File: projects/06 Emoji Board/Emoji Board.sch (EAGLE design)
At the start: 25 parts, among them M2 MAX7219, U2 ATMEGA8A-AU-TQFP32, Y1 16MHZ

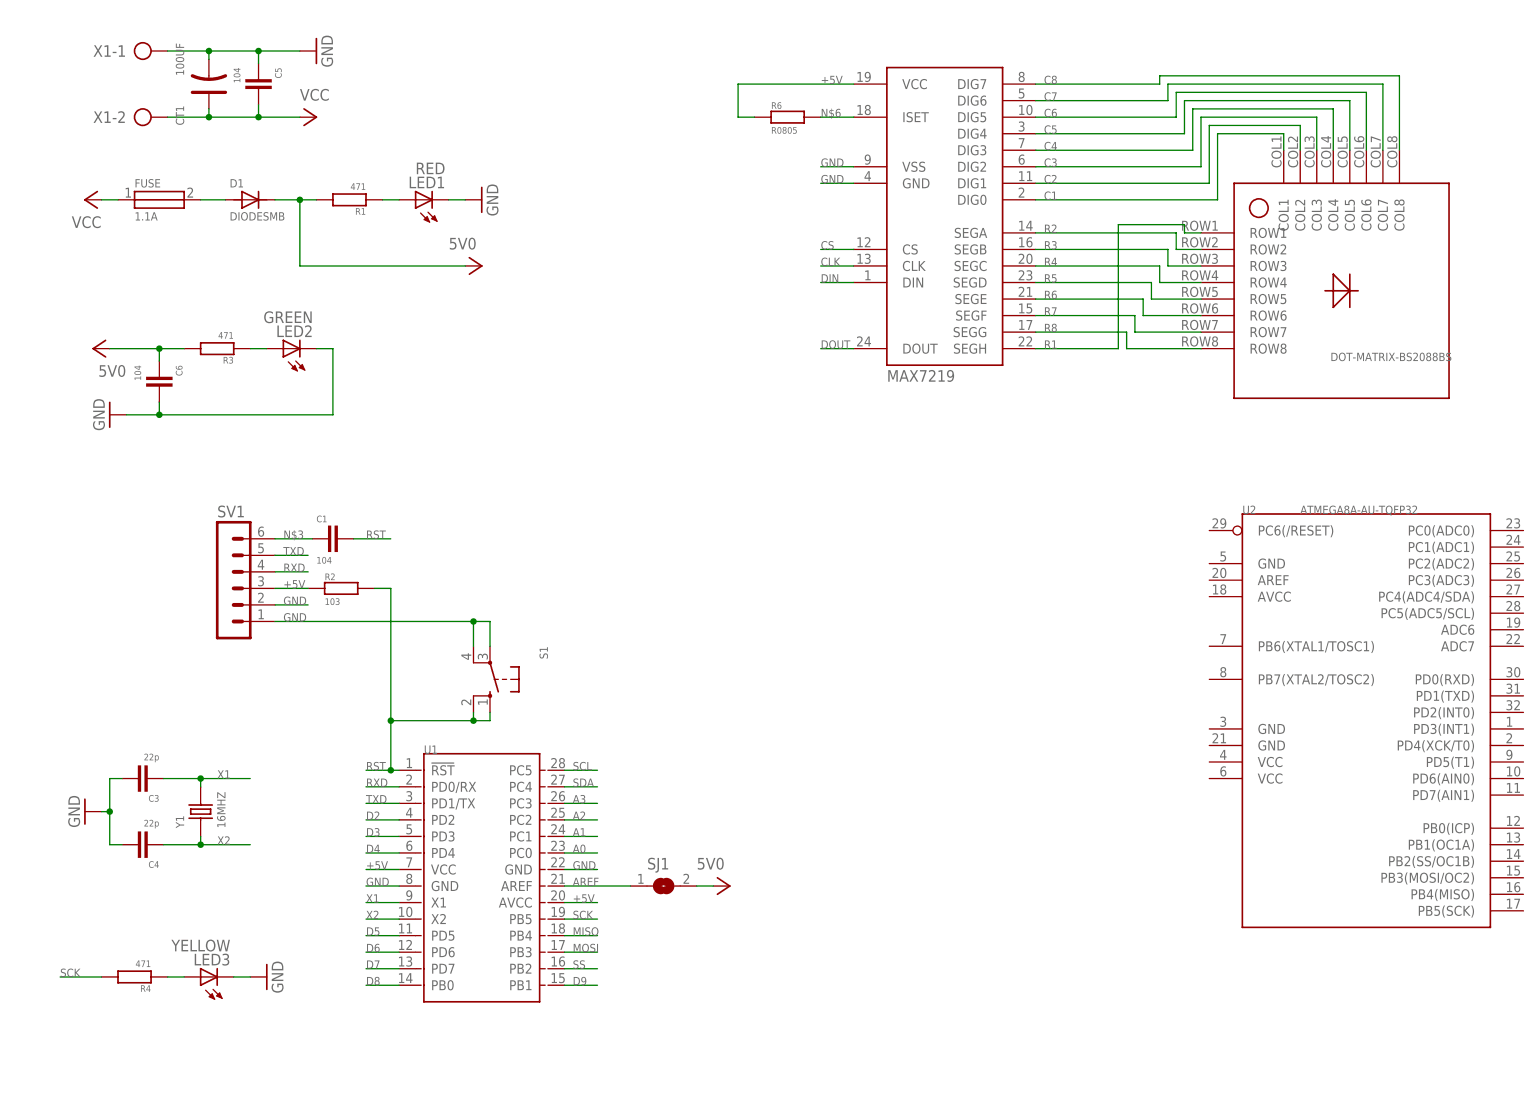
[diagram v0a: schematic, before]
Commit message: 2020.06.24.04
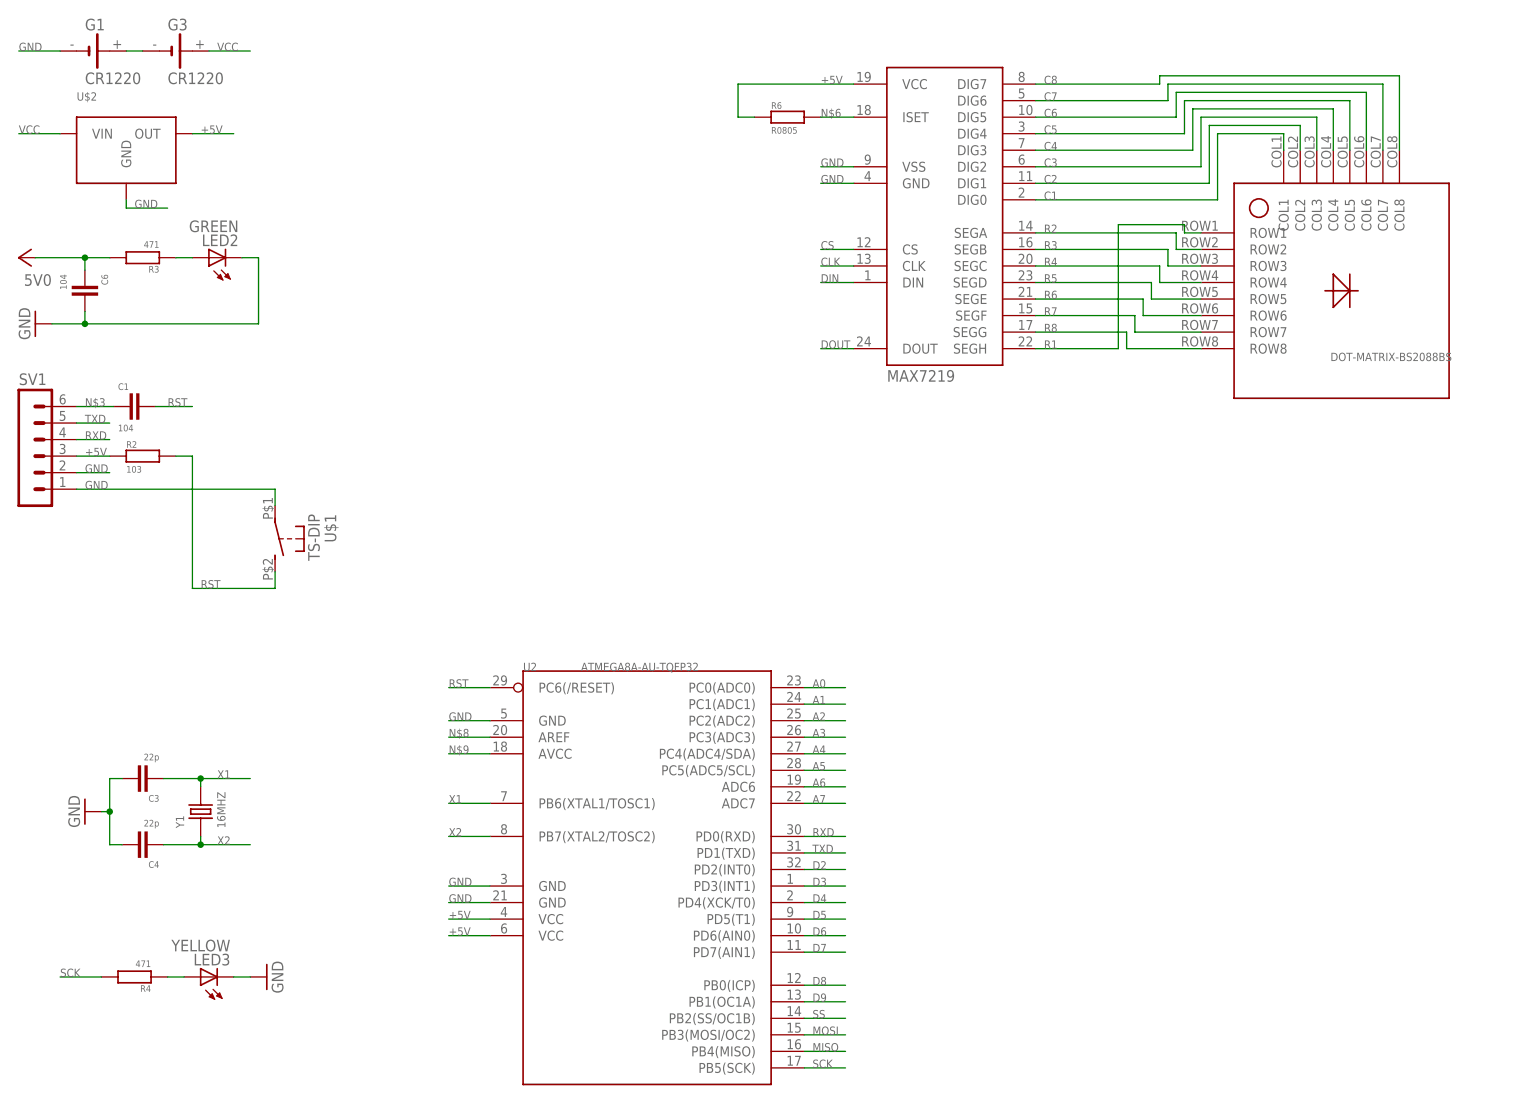
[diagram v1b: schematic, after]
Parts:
- removed C5: 104, RCLDA:C0805
- removed CT1: 100UF, RCLDA:ALUMINUM-SMD-100UF-50V(D6.0-H6.0MM)
- removed D1: DIODESMB, RCLDA:DIODESMB
- removed FUSE: 1.1A, RCLDA:FUSE0805
- removed LED1: RED, Display:LEDCHIPLED_0805
- removed R1: 471, RCLDA:R0805
- removed S1: (no value), Button:TS-DIP-4.54.5
- removed SJ1: (no value), Jumper:SJ
- removed U1: (no value), Chip:MCU-ATMEGA328P-PU(DIP28)
- removed X1: (no value), Connector:AK500/2
- added G1, G3: CR1220, Power:CR1220
- added U$1: TS-DIP, Button:TS-DIP
- added U$2: AMS1117-5V0SOT22, Chip:AMS1117-5V0SOT22
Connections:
- removed net AREF: SJ1.1, U1.AREF
- removed net N$4: LED1.A, R1.1
- removed net SCL: U1.PC5
- removed net SDA: U1.PC4
- new net A4: U2.PC4(ADC4/SDA)
- new net A5: U2.PC5(ADC5/SCL)
- new net A6: U2.ADC6
- new net A7: U2.ADC7
- new net N$8: U2.AREF
- new net N$9: U2.AVCC
- net +5V: now also U$2.OUT, U2.VCC@1, U2.VCC@2; no longer D1.1, R1.2, SJ1.2, U1.AVCC, U1.VCC
- net A0: now also U2.PC0(ADC0); no longer U1.PC0
- net A1: now also U2.PC1(ADC1); no longer U1.PC1
- net A2: now also U2.PC2(ADC2); no longer U1.PC2
- net A3: now also U2.PC3(ADC3); no longer U1.PC3
- net D2: now also U2.PD2(INT0); no longer U1.PD2
- net D3: now also U2.PD3(INT1); no longer U1.PD3
- net D4: now also U2.PD4(XCK/T0); no longer U1.PD4
- net D5: now also U2.PD5(T1); no longer U1.PD5
- net D6: now also U2.PD6(AIN0); no longer U1.PD6
- net D7: now also U2.PD7(AIN1); no longer U1.PD7
- net D8: now also U2.PB0(ICP); no longer U1.PB0
- net D9: now also U2.PB1(OC1A); no longer U1.PB1
- net GND: now also G1.-, U$1.P, U$2.GND, U2.GND, U2.GND@1, U2.GND@2; no longer C5.2, CT1.-, LED1.C, S1.P, S1.P1, U1.GND@1, U1.GND@2, X1-1.KL
- net MISO: now also U2.PB4(MISO); no longer U1.PB4
- net MOSI: now also U2.PB3(MOSI/OC2); no longer U1.PB3
- net N$2: now also G1.+, G3.-; no longer D1.2, FUSE.P$2
- net RST: now also U$1.S, U2.PC6(/RESET); no longer S1.S, S1.S1, U1.!RST
- net RXD: now also U2.PD0(RXD); no longer U1.PD0/RX
- net SCK: now also U2.PB5(SCK); no longer U1.PB5
- net SS: now also U2.PB2(SS/OC1B); no longer U1.PB2
- net TXD: now also U2.PD1(TXD); no longer U1.PD1/TX
- net VCC: now also G3.+, U$2.VIN; no longer C5.1, CT1.+, FUSE.P$1, X1-2.KL
- net X1: now also U2.PB6(XTAL1/TOSC1); no longer U1.X1
- net X2: now also U2.PB7(XTAL2/TOSC2); no longer U1.X2
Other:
- moved on the sheet: C1, C6, LED2, R2, R3, SV1, U2
